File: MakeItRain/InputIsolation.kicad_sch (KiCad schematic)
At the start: 9 parts, among them IC2 LTV-846S

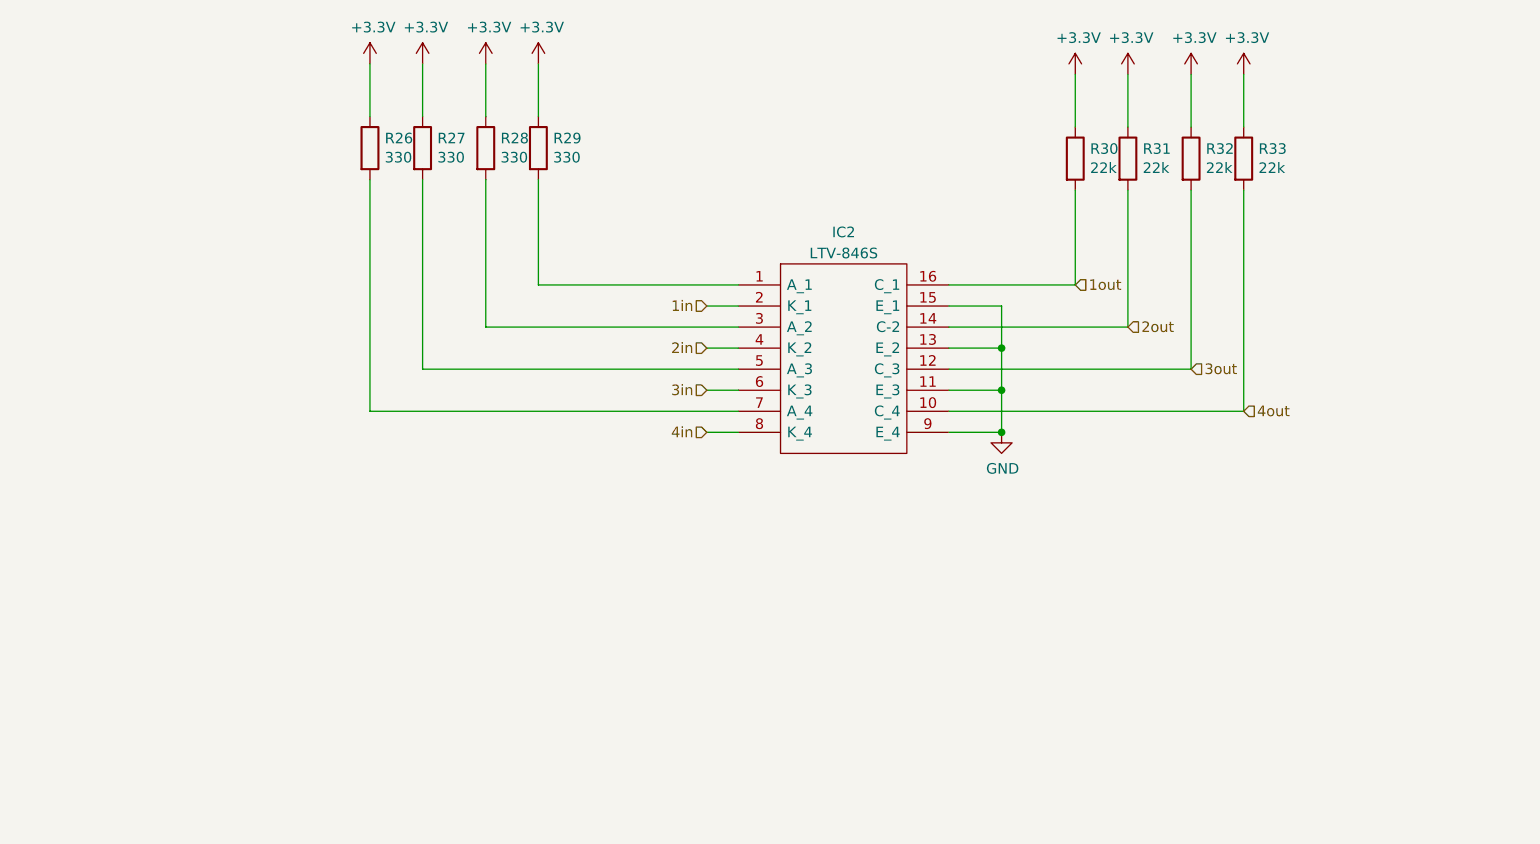
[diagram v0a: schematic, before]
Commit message: imput redesign
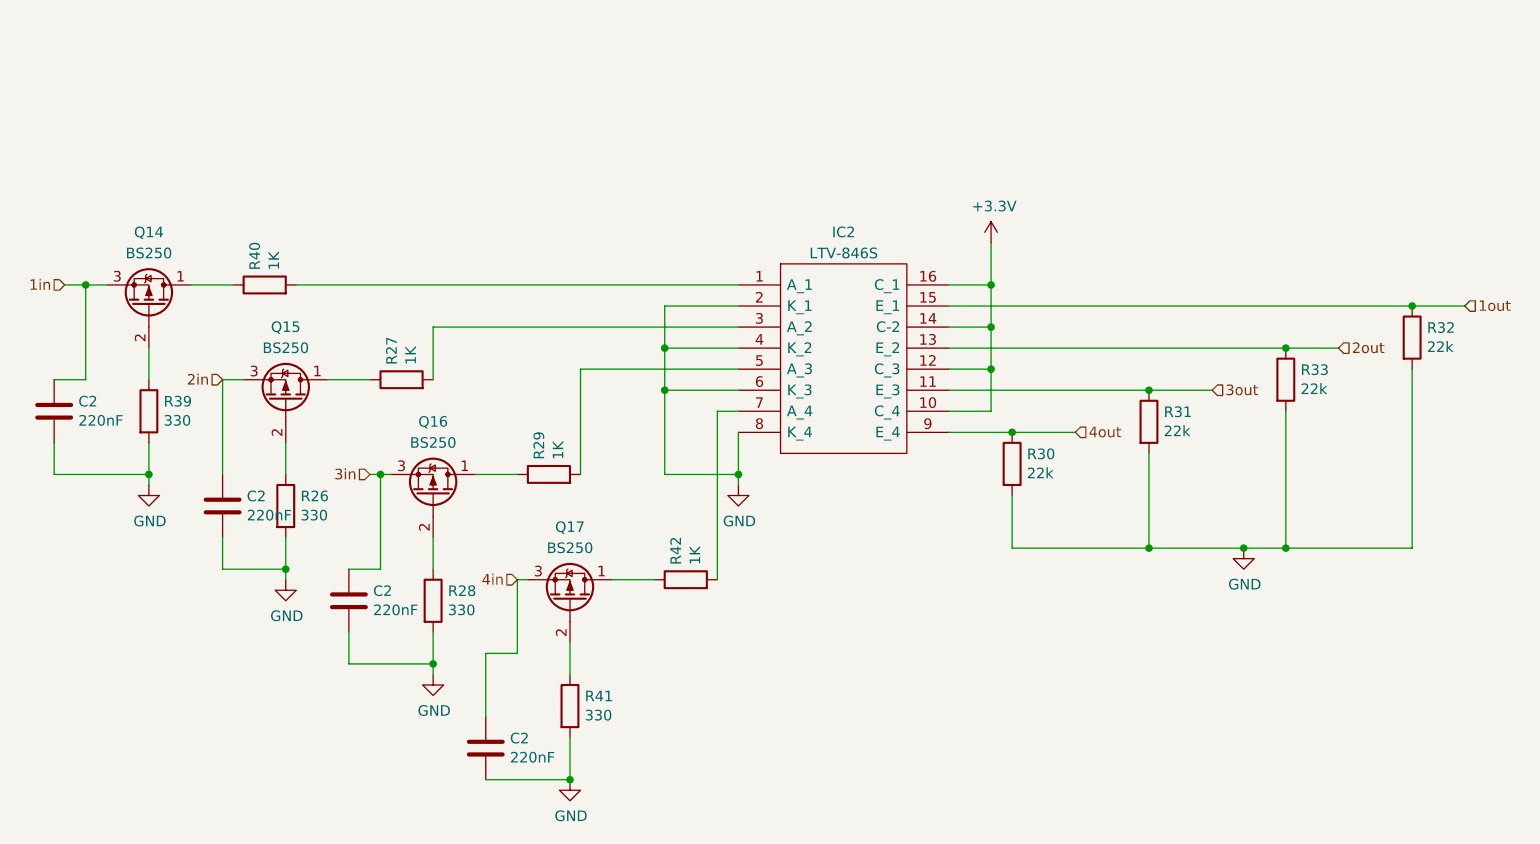
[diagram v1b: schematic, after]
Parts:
- added C2 (x4): 220nF, Capacitor_THT:C_Disc_D5.1mm_W3.2mm_P5.00mm, symbol Device:C
- added Q14, Q15, Q16, Q17: BS250, Package_TO_SOT_THT:TO-92_Inline, symbol Transistor_FET:BS250
- added R39, R41: 330, Resistor_THT:R_Axial_DIN0207_L6.3mm_D2.5mm_P2.54mm_Vertical, symbol Device:R
- added R40, R42: 1K, Resistor_THT:R_Axial_DIN0207_L6.3mm_D2.5mm_P2.54mm_Vertical, symbol Device:R
- R27, R29: value 330 -> 1K
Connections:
- net +3V3: now also IC2.10 (C_4), IC2.12 (C_3), IC2.14 (C-2), IC2.16 (C_1); no longer R26.1, R27.1, R28.1, R29.1, R30.1, R31.1, R32.1, R33.1
- net 1in: now also C2.1, Q14.3 (S); no longer IC2.2 (K_1)
- net 1out: now also IC2.15 (E_1), R32.1; no longer IC2.16 (C_1), R30.2
- net 2in: now also C2.1, Q15.3 (S); no longer IC2.4 (K_2)
- net 2out: now also IC2.13 (E_2), R33.1; no longer IC2.14 (C-2), R31.2
- net 3in: now also C2.1, Q16.3 (S); no longer IC2.6 (K_3)
- net 3out: now also IC2.11 (E_3), R31.1; no longer IC2.12 (C_3), R32.2
- net 4in: now also C2.1, Q17.3 (S); no longer IC2.8 (K_4)
- net 4out: now also IC2.9 (E_4), R30.1; no longer IC2.10 (C_4), R33.2
- net GND: now also IC2.2 (K_1), IC2.4 (K_2), IC2.6 (K_3), IC2.8 (K_4), R26.2, R28.2, R30.2, R31.2, R32.2, R33.2, C2.2, C2.2, C2.2, C2.2, R39.2, R41.2; no longer IC2.11 (E_3), IC2.13 (E_2), IC2.15 (E_1), IC2.9 (E_4)
- net at IC2.7 (A_4): now also R42.2; no longer R26.2
- net at R27.2: now also IC2.3 (A_2); no longer IC2.5 (A_3)
- net at IC2.1 (A_1): now also R40.2; no longer R29.2
- new net: Q14.1 (D), R40.1
- new net: Q14.2 (G), R39.1
- new net: Q15.1 (D), R27.1
- new net: Q16.1 (D), R29.1
- new net: Q16.2 (G), R28.1
- new net: Q17.2 (G), R41.1
- new net: Q17.1 (D), R42.1
- new net: Q15.2 (G), R26.1
- new net: IC2.5 (A_3), R29.2
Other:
- moved on the sheet: R30, R31, R32, R33
